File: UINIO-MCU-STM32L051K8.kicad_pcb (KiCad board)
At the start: 2 copper layers, 48.4 x 20.5 mm, 32 parts, among them J1 Conn_01x14_Male, J2 Conn_01x14_Male, J3 Conn_01x04_Male, SW1 SW_Push, SW2 SW_Push, U1 ME6211C33M5G-N, U2 W25Q128JVSSIQ, U3 STM32L051K8U6, Y1 FC135-32.768

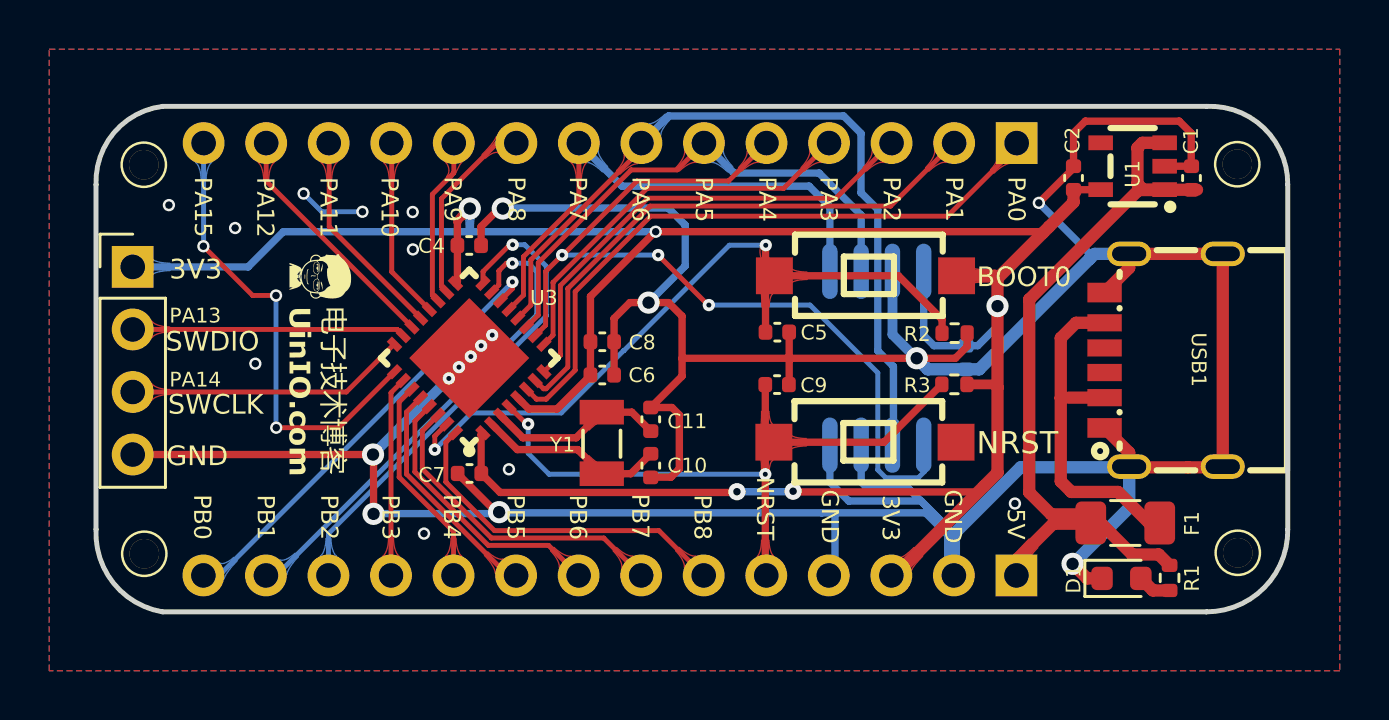
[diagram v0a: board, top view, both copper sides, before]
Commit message: Update PCB.
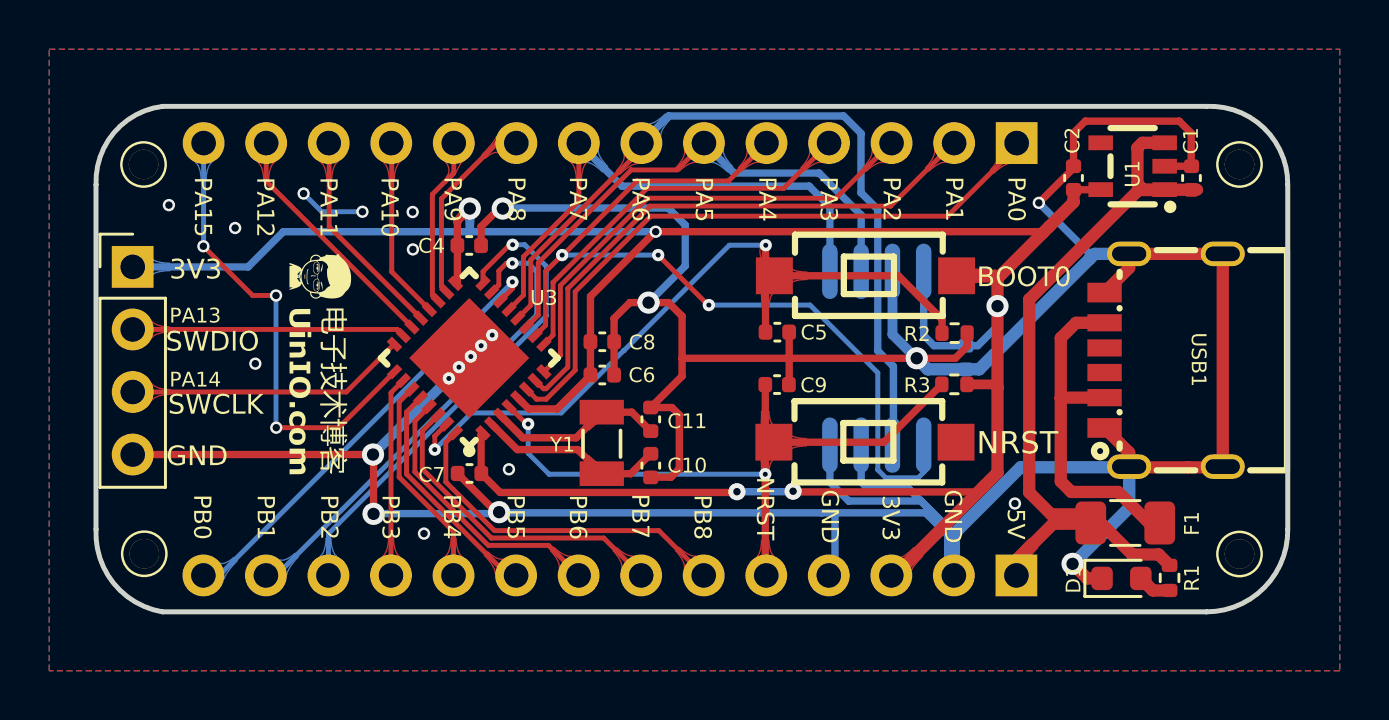
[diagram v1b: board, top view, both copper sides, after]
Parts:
- moved Hole4 0.09 mm to (175.0, 91.8)
- moved Hole3 0.09 mm to (175.0, 107.6)

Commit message: Fix bug.
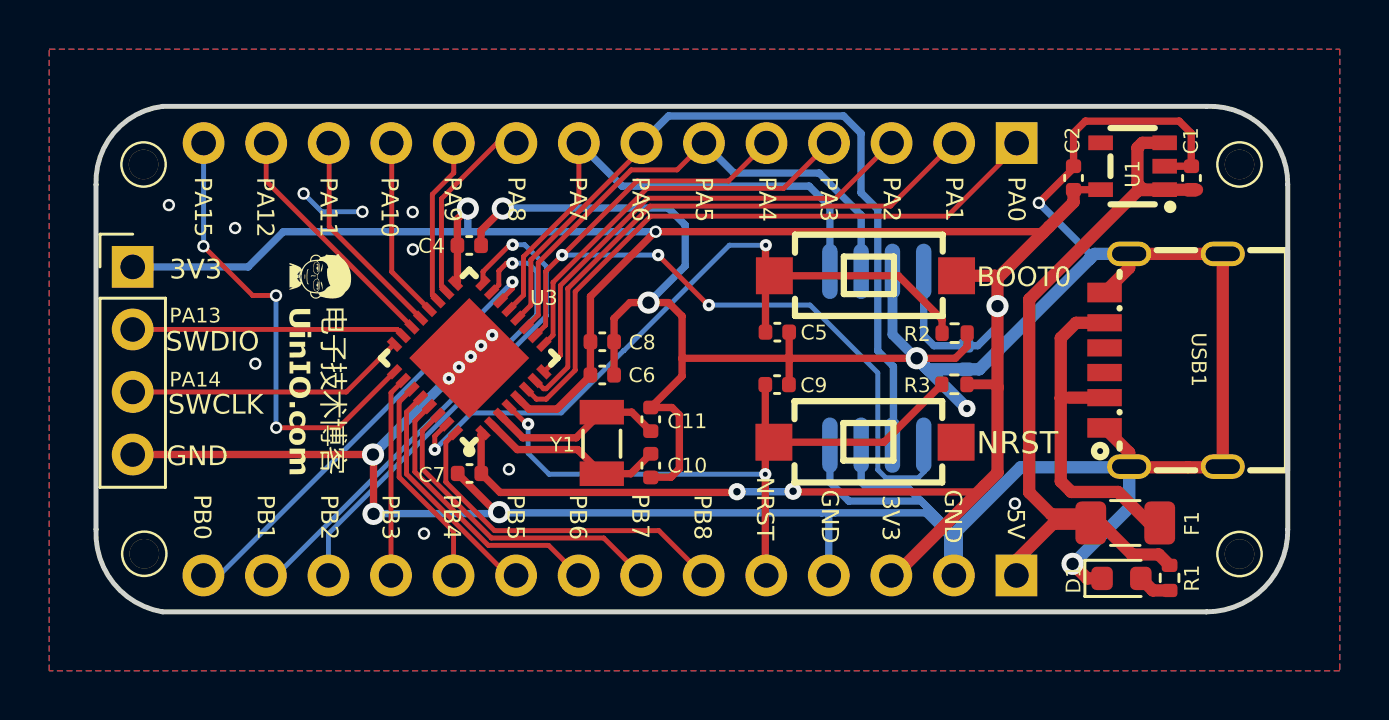
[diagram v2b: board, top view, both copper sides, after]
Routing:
- net GND: track 175.7 -> 178.6 mm, vias 23 -> 24

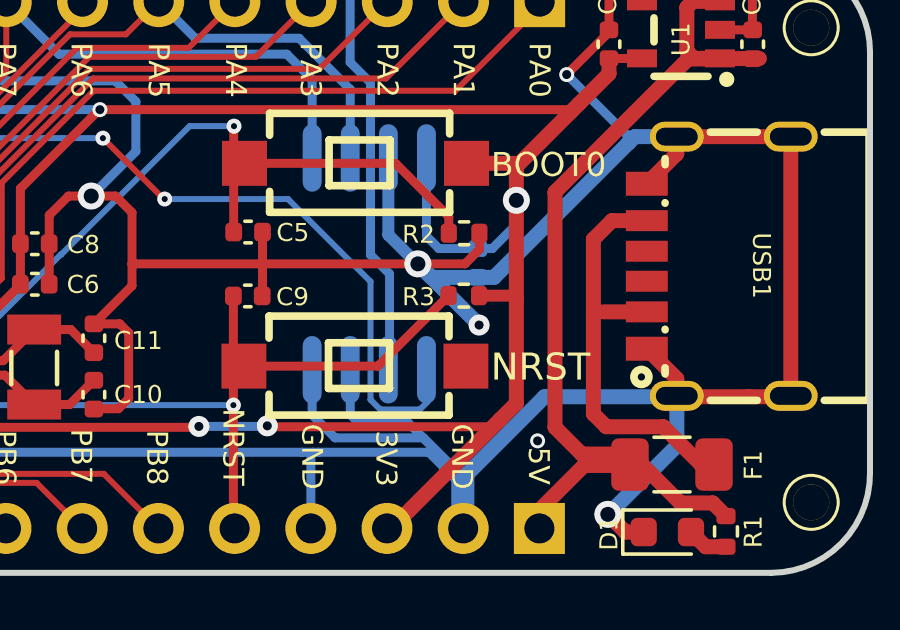
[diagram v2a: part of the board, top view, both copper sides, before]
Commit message: update
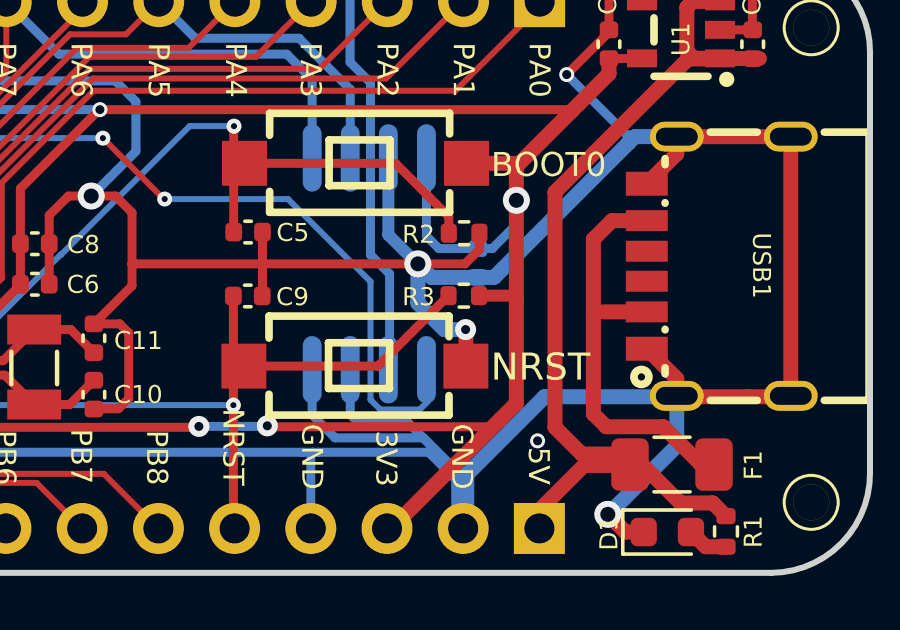
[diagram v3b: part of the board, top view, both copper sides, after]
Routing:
- net GND: track 178.6 -> 180.2 mm
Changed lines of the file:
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@@
   (segment (start 172.59 90.05) (end 173.08 90.54) (width 0.3) (layer "F.Cu") (net 1))
   (segment (start 170.56 96.01) (end 169.56 97.01) (width 0.5) (layer "F.Cu") (net 1))
+  (segment (start 163.52 101.87) (end 163.53 101.88) (width 0.5) (layer "F.Cu") (net 1))
   (segment (start 174.21 104.11) (end 172.95 104.11) (width 0.5) (layer "F.Cu") (net 1))
   (segment (start 152.29 104.17) (end 151.95 104.51) (width 0.3) (layer "F.Cu") (net 1))
@@
   (segment (start 156.78 99.73) (end 156.75 99.7) (width 0.3) (layer "F.Cu") (net 1))
   (segment (start 152.4 100.41) (end 152.4 99.69) (width 0.3) (layer "F.Cu") (net 1))
+  (segment (start 163.53 101.88) (end 163.53 103.09) (width 0.5) (layer "F.Cu") (net 1))
   (segment (start 156.75 99.76) (end 156.75 100.74) (width 0.3) (layer "F.Cu") (net 1))
   (segment (start 163.5 99.68) (end 161.93 99.68) (width 0.3) (layer "F.Cu") (net 1))
@@
   (via (at 134.25 94.39) (size 0.5) (drill 0.3) (layers "F.Cu" "B.Cu") (free) (net 1))
   (via (at 139.42 93.73) (size 0.5) (drill 0.3) (layers "F.Cu" "B.Cu") (free) (net 1))
-  (via (at 163.97 101.72) (size 0.7) (drill 0.3) (layers "F.Cu" "B.Cu") (net 1))
+  (via (at 163.52 101.87) (size 0.7) (drill 0.3) (layers "F.Cu" "B.Cu") (net 1))
   (via (at 168.26 108.03) (size 0.9) (drill 0.5) (layers "F.Cu" "B.Cu") (net 1))
   (via (at 144.24 99.17) (size 0.5) (drill 0.2) (layers "F.Cu" "B.Cu") (remove_unused_layers) (net 1))
@@
   (segment (start 164.47 100.13) (end 168.955 95.645) (width 0.5) (layer "B.Cu") (net 1))
   (segment (start 162.11 105.48) (end 163.19 106.56) (width 0.3) (layer "B.Cu") (net 1))
-  (segment (start 163.97 101.72) (end 161.93 99.68) (width 0.5) (layer "B.Cu") (net 1))
   (segment (start 144.69 98.74) (end 142.93 100.5) (width 0.4) (layer "B.Cu") (net 1))
   (segment (start 159.95 104.98) (end 161.61 104.98) (width 0.3) (layer "B.Cu") (net 1))
@@
   (segment (start 139.85 103.59) (end 139.85 103.58) (width 0.4) (layer "B.Cu") (net 1))
   (segment (start 139.87 106) (end 139.88 105.99) (width 0.3) (layer "B.Cu") (net 1))
+  (segment (start 162.81 101.87) (end 161.93 100.99) (width 0.5) (layer "B.Cu") (net 1))
   (segment (start 170.41 104.11) (end 166.15 104.11) (width 0.5) (layer "B.Cu") (net 1))
   (segment (start 159.17 105.48) (end 162.11 105.48) (width 0.3) (layer "B.Cu") (net 1))
@@
   (segment (start 163.56 106.7) (end 163.56 108.38) (width 0.5) (layer "B.Cu") (net 1))
   (segment (start 170.56 105.75) (end 170.56 104.08) (width 0.5) (layer "B.Cu") (net 1))
+  (segment (start 163.52 101.87) (end 162.81 101.87) (width 0.5) (layer "B.Cu") (net 1))
   (segment (start 158.43 105.96) (end 158.61 105.96) (width 0.3) (layer "B.Cu") (net 1))
   (segment (start 158.08 105.96) (end 158.43 105.96) (width 0.3) (layer "B.Cu") (net 1))
@@
   (segment (start 139.85 103.58) (end 142.93 100.5) (width 0.4) (layer "B.Cu") (net 1))
   (segment (start 163.93 100.13) (end 164.47 100.13) (width 0.5) (layer "B.Cu") (net 1))
+  (segment (start 161.93 100.99) (end 161.93 99.68) (width 0.5) (layer "B.Cu") (net 1))
   (segment (start 158.405 103.21) (end 158.405 104.715) (width 0.3) (layer "B.Cu") (net 1))
   (segment (start 152.53 95.93) (end 151.04 97.42) (width 0.3) (layer "B.Cu") (net 1))
